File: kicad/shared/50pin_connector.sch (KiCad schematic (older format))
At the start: 1 part, among them P5 CONN_02X25

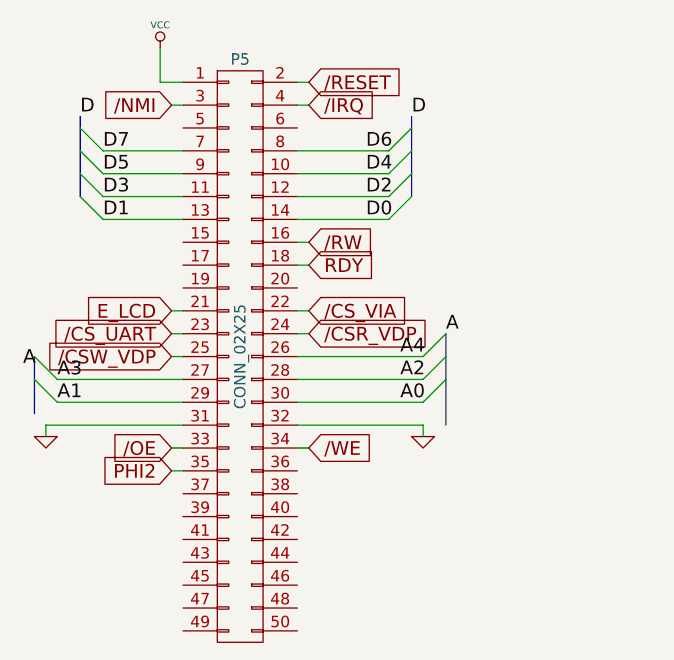
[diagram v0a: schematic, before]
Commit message: connector
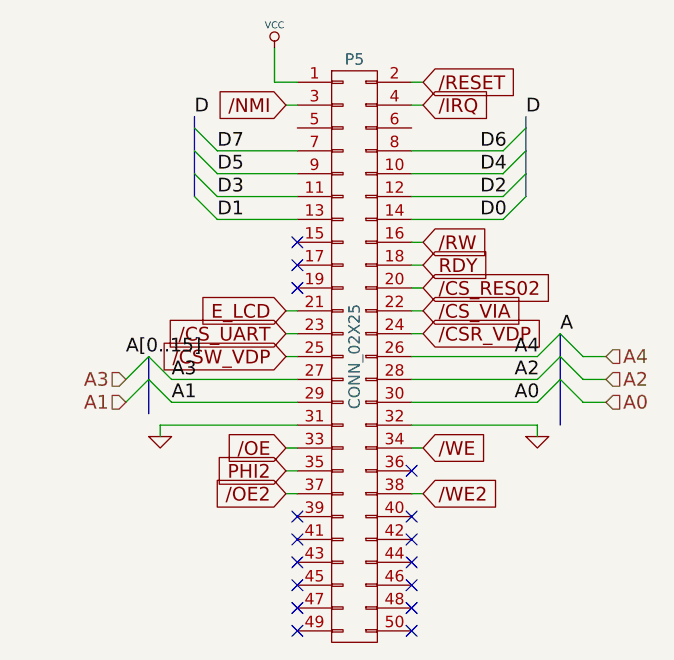
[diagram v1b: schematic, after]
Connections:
- net /CS_RES02: now reaches P5.20 (P20)
- net /OE2: now reaches P5.37 (P37)
- net /WE2: now reaches P5.38 (P38)
- no-connect marks 0 -> 16
